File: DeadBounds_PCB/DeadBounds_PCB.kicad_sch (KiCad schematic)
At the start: 0 parts

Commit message: Test
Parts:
- added U1: MSPM0G3507SPMR, symbol DeadBounds_Symbols:MSPM0G3507SPMR
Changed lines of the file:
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@@
 	(generator_version "10.0")
 	(paper "A4")
+	(symbol
+		(lib_id "DeadBounds_Symbols:MSPM0G3507SPMR")
+		(at 115.57 25.4 0)
+		(unit 1)
+		(body_style 1)
+		(exclude_from_sim no)
+		(in_bom yes)
+		(on_board no)
+		(in_pos_files yes)
+		(dnp no)
+		(fields_autoplaced yes)
+		(property "Reference" "U1"
+			(at 148.5392 129.54 0)
+			(show_name no)
+			(do_not_autoplace no)
+			(effects
+				(font
+					(size 1.524 1.524)
+				)
+			)
+		)
+		(property "Value" "MSPM0G3507SPMR"
+			(at 148.5392 132.08 0)
+			(show_name no)
+			(do_not_autoplace no)
+			(effects
+				(font
+					(size 1.524 1.524)
+				)
+			)
+		)
+		(property "Footprint" ""
+			(at 165.354 14.732 0)
+			(hide yes)
+			(show_name no)
+			(do_not_autoplace no)
+			(effects
+				(font
+					(size 1.27 1.27)
+					(italic yes)
+				)
+			)
+		)
+		(property "Datasheet" ""
+			(at 135.382 2.032 0)
+			(hide yes)
+			(show_name no)
+			(do_not_autoplace no)
+			(effects
+				(font
+					(size 1.27 1.27)
+					(italic yes)
+				)
+			)
+		)
+		(property "Description" ""
+			(at 115.57 25.4 0)
+			(hide yes)
+			(show_name no)
+			(do_not_autoplace no)
+			(effects
+				(font
+					(size 1.27 1.27)
+				)
+			)
+		)
+		(pin "3"
+		)
+		(pin "18"
+		)
+		(pin "9"
+		)
+		(pin "12"
+		)
+		(pin "13"
+		)
+		(pin "15"
+		)
+		(pin "14"
+		)
+		(pin "6"
+		)
+		(pin "17"
+		)
+		(pin "7"
+		)
+		(pin "25"
+		)
+		(pin "2"
+		)
+		(pin "10"
+		)
+		(pin "11"
+		)
+		(pin "5"
+		)
+		(pin "16"
+		)
+		(pin "21"
+		)
+		(pin "23"
+		)
+		(pin "1"
+		)
+		(pin "19"
+		)
+		(pin "8"
+		)
+		(pin "24"
+		)
+		(pin "31"
+		)
+		(pin "4"
+		)
+		(pin "27"
+		)
+		(pin "47"
+		)
+		(pin "20"
+		)
+		(pin "29"
+		)
+		(pin "40"
+		)
+		(pin "33"
+		)
+		(pin "44"
+		)
+		(pin "35"
+		)
+		(pin "37"
+		)
+		(pin "22"
+		)
+		(pin "38"
+		)
+		(pin "39"
+		)
+		(pin "41"
+		)
+		(pin "42"
+		)
+		(pin "45"
+		)
+		(pin "32"
+		)
+		(pin "46"
+		)
+		(pin "58"
+		)
+		(pin "64"
+		)
+		(pin "30"
+		)
+		(pin "28"
+		)
+		(pin "26"
+		)
+		(pin "34"
+		)
+		(pin "36"
+		)
+		(pin "43"
+		)
+		(pin "52"
+		)
+		(pin "54"
+		)
+		(pin "57"
+		)
+		(pin "60"
+		)
+		(pin "55"
+		)
+		(pin "53"
+		)
+		(pin "59"
+		)
+		(pin "62"
+		)
+		(pin "51"
+		)
+		(pin "49"
+		)
+		(pin "50"
+		)
+		(pin "56"
+		)
+		(pin "61"
+		)
+		(pin "63"
+		)
+		(pin "48"
+		)
+		(instances
+			(project "DeadBounds_PCB"
+				(path "/c652495f-dd42-4f45-9891-1e05b67942c0"
+					(reference "U1")
+					(unit 1)
+				)
+			)
+		)
+	)
 	(sheet_instances
 		(path "/"

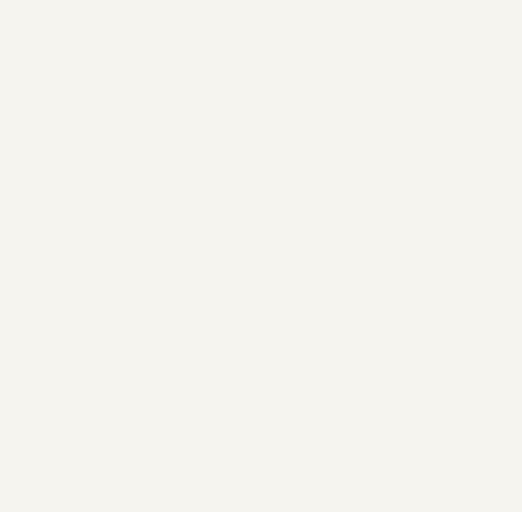
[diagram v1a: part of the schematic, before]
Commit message: Test 2
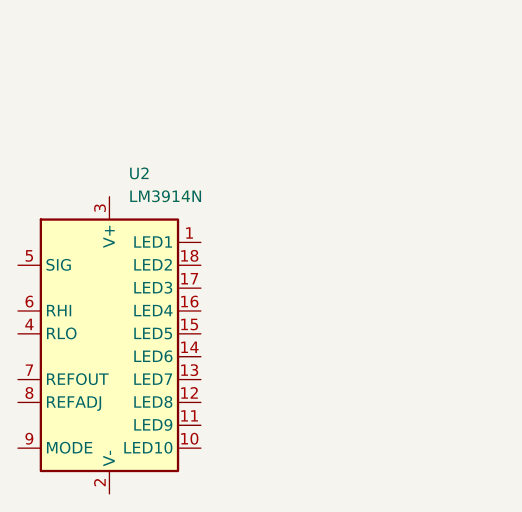
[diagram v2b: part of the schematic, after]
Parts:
- added U2: LM3914N, Package_DIP:DIP-18_W7.62mm, symbol Driver_LED:LM3914N
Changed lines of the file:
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@@
+		)
+	)
+	(symbol
+		(lib_id "Driver_LED:LM3914N")
+		(at 48.26 121.92 0)
+		(unit 1)
+		(body_style 1)
+		(exclude_from_sim no)
+		(in_bom yes)
+		(on_board yes)
+		(in_pos_files yes)
+		(dnp no)
+		(fields_autoplaced yes)
+		(property "Reference" "U2"
+			(at 50.4033 104.14 0)
+			(show_name no)
+			(do_not_autoplace no)
+			(effects
+				(font
+					(size 1.27 1.27)
+				)
+				(justify left)
+			)
+		)
+		(property "Value" "LM3914N"
+			(at 50.4033 106.68 0)
+			(show_name no)
+			(do_not_autoplace no)
+			(effects
+				(font
+					(size 1.27 1.27)
+				)
+				(justify left)
+			)
+		)
+		(property "Footprint" "Package_DIP:DIP-18_W7.62mm"
+			(at 48.26 121.92 0)
+			(hide yes)
+			(show_name no)
+			(do_not_autoplace no)
+			(effects
+				(font
+					(size 1.27 1.27)
+				)
+			)
+		)
+		(property "Datasheet" "https://www.ti.com/lit/ds/symlink/lm3914.pdf"
+			(at 48.26 121.92 0)
+			(hide yes)
+			(show_name no)
+			(do_not_autoplace no)
+			(effects
+				(font
+					(size 1.27 1.27)
+				)
+			)
+		)
+		(property "Description" "10 LED Dot/Bar Display Driver, DIP-18"
+			(at 48.26 121.92 0)
+			(hide yes)
+			(show_name no)
+			(do_not_autoplace no)
+			(effects
+				(font
+					(size 1.27 1.27)
+				)
+			)
+		)
+		(pin "6"
+		)
+		(pin "10"
+		)
+		(pin "1"
+		)
+		(pin "4"
+		)
+		(pin "8"
+		)
+		(pin "13"
+		)
+		(pin "14"
+		)
+		(pin "2"
+		)
+		(pin "5"
+		)
+		(pin "7"
+		)
+		(pin "15"
+		)
+		(pin "9"
+		)
+		(pin "16"
+		)
+		(pin "11"
+		)
+		(pin "3"
+		)
+		(pin "17"
+		)
+		(pin "12"
+		)
+		(pin "18"
+		)
+		(instances
+			(project "DeadBounds_PCB"
+				(path "/c652495f-dd42-4f45-9891-1e05b67942c0"
+					(reference "U2")
+					(unit 1)
+				)
+			)
 		)
 	)
